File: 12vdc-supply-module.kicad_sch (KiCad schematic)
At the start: 1 part

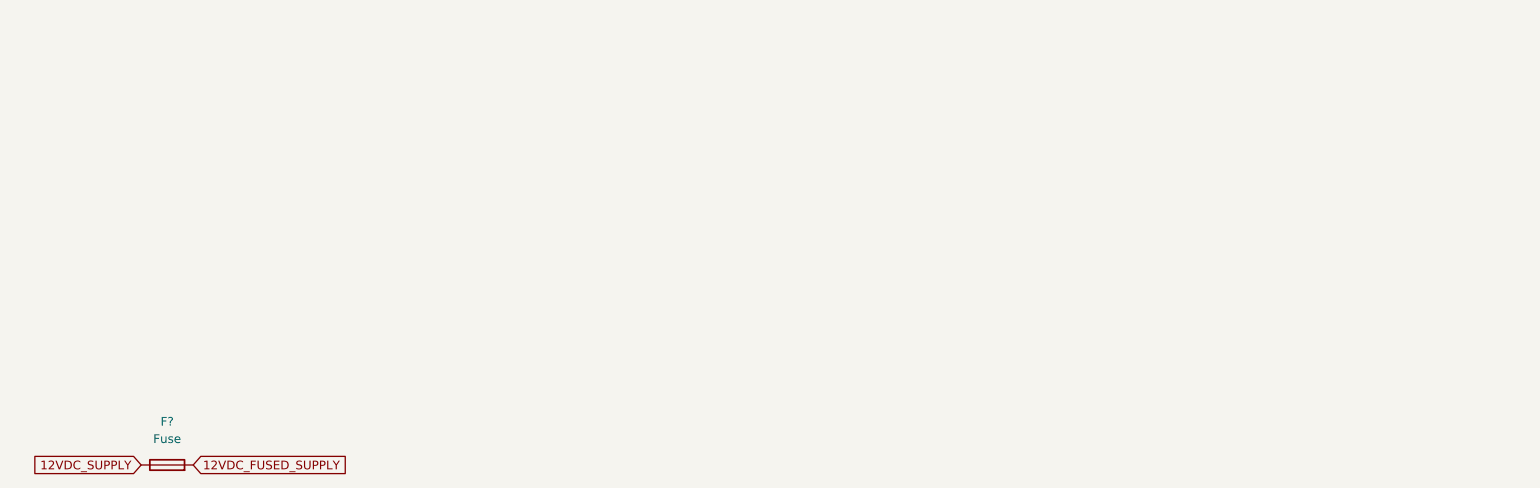
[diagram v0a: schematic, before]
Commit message: Draft 5VDC Supply Schematic
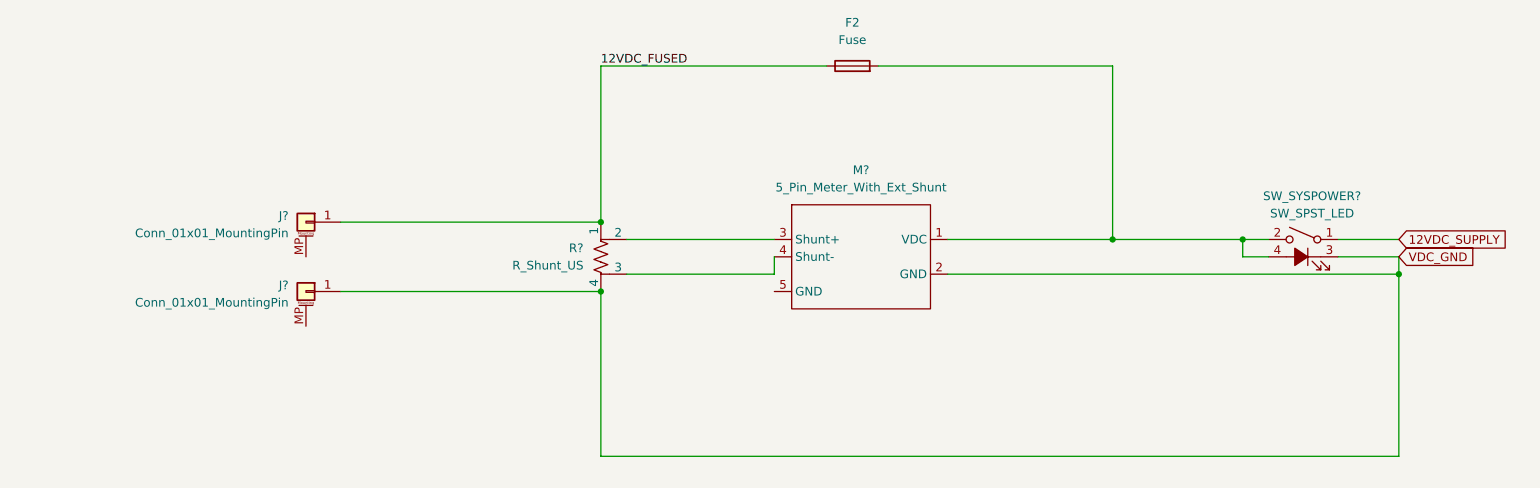
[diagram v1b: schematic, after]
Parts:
- added J? (x2): Conn_01x01_MountingPin, symbol Connector_Generic_MountingPin:Conn_01x01_MountingPin
- added M?: 5_Pin_Meter_With_Ext_Shunt, symbol bvm-library:5_Pin_Meter_With_Ext_Shunt
- added R?: R_Shunt_US, symbol Device:R_Shunt_US
- added SW_SYSPOWER?: SW_SPST_LED, symbol Switch:SW_SPST_LED
- gave numbers to parts that had none: 1
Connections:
- net 12VDC_SUPPLY: now also SW_SYSPOWER?.1; no longer F2.1
- net 12VDC_FUSED_SUPPLY: no longer names the net of F2.2
- net 12VDC_FUSED_SUPPLY: now also M?.1 (VDC), SW_SYSPOWER?.2, SW_SYSPOWER?.4 (A)
- new net: M?.3 (Shunt+), R?.2
- new net: M?.4 (Shunt-), R?.3
- new net 12VDC_FUSED: F2.1, J?.1 (Pin_1), R?.1
- new net VDC_GND: J?.1 (Pin_1), M?.2 (GND), R?.4, SW_SYSPOWER?.3 (K)
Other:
- moved on the sheet: F2
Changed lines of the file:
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@@
     (company "eatmellc")
   )
-  (global_label "12VDC_SUPPLY" (shape input) (at 68.58 82.55 180) (fields_autoplaced)
-    (effects (font (size 1.27 1.27)) (justify right))
-    (property "Intersheet References" "${INTERSHEET_REFS}" (id 0) (at 51.955 82.4706 0)
-      (effects (font (size 1.27 1.27)) (justify right))
-    )
+  (junction (at 135.89 46.99) (diameter 0) (color 0 0 0 0)
   )
-  (global_label "12VDC_FUSED_SUPPLY" (shape input) (at 76.2 82.55 0) (fields_autoplaced)
+  (junction (at 135.89 57.15) (diameter 0) (color 0 0 0 0)
+  )
+  (junction (at 229.87 49.53) (diameter 0) (color 0 0 0 0)
+  )
+  (junction (at 210.82 49.53) (diameter 0) (color 0 0 0 0)
+  )
+  (junction (at 252.73 54.61) (diameter 0) (color 0 0 0 0)
+  )
+  (wire (pts (xy 229.87 52.07) (xy 233.68 52.07))
+    (stroke (width 0) (type default) (color 0 0 0 0))
+  )
+  (wire (pts (xy 135.89 24.13) (xy 135.89 46.99))
+    (stroke (width 0) (type default) (color 0 0 0 0))
+  )
+  (wire (pts (xy 139.7 49.53) (xy 161.29 49.53))
+    (stroke (width 0) (type default) (color 0 0 0 0))
+  )
+  (wire (pts (xy 210.82 49.53) (xy 210.82 24.13))
+    (stroke (width 0) (type default) (color 0 0 0 0))
+  )
+  (wire (pts (xy 252.73 52.07) (xy 252.73 54.61))
+    (stroke (width 0) (type default) (color 0 0 0 0))
+  )
+  (wire (pts (xy 135.89 81.28) (xy 135.89 57.15))
+    (stroke (width 0) (type default) (color 0 0 0 0))
+  )
+  (wire (pts (xy 161.29 54.61) (xy 161.29 52.07))
+    (stroke (width 0) (type default) (color 0 0 0 0))
+  )
+  (wire (pts (xy 233.68 49.53) (xy 229.87 49.53))
+    (stroke (width 0) (type default) (color 0 0 0 0))
+  )
+  (wire (pts (xy 252.73 54.61) (xy 252.73 81.28))
+    (stroke (width 0) (type default) (color 0 0 0 0))
+  )
+  (wire (pts (xy 97.79 46.99) (xy 135.89 46.99))
+    (stroke (width 0) (type default) (color 0 0 0 0))
+  )
+  (wire (pts (xy 229.87 49.53) (xy 229.87 52.07))
+    (stroke (width 0) (type default) (color 0 0 0 0))
+  )
+  (wire (pts (xy 252.73 52.07) (xy 243.84 52.07))
+    (stroke (width 0) (type default) (color 0 0 0 0))
+  )
+  (wire (pts (xy 161.29 54.61) (xy 139.7 54.61))
+    (stroke (width 0) (type default) (color 0 0 0 0))
+  )
+  (wire (pts (xy 252.73 49.53) (xy 243.84 49.53))
+    (stroke (width 0) (type default) (color 0 0 0 0))
+  )
+  (wire (pts (xy 252.73 81.28) (xy 135.89 81.28))
+    (stroke (width 0) (type default) (color 0 0 0 0))
+  )
+  (wire (pts (xy 210.82 49.53) (xy 186.69 49.53))
+    (stroke (width 0) (type default) (color 0 0 0 0))
+  )
+  (wire (pts (xy 168.91 24.13) (xy 135.89 24.13))
+    (stroke (width 0) (type default) (color 0 0 0 0))
+  )
+  (wire (pts (xy 186.69 54.61) (xy 252.73 54.61))
+    (stroke (width 0) (type default) (color 0 0 0 0))
+  )
+  (wire (pts (xy 210.82 24.13) (xy 176.53 24.13))
+    (stroke (width 0) (type default) (color 0 0 0 0))
+  )
+  (wire (pts (xy 97.79 57.15) (xy 135.89 57.15))
+    (stroke (width 0) (type default) (color 0 0 0 0))
+  )
+  (wire (pts (xy 229.87 49.53) (xy 210.82 49.53))
+    (stroke (width 0) (type default) (color 0 0 0 0))
+  )
+  (label "12VDC_FUSED" (at 135.89 24.13 0)
+    (effects (font (size 1.27 1.27)) (justify left bottom))
+  )
+  (global_label "VDC_GND" (shape input) (at 252.73 52.07 0) (fields_autoplaced)
     (effects (font (size 1.27 1.27)) (justify left))
-    (property "Intersheet References" "${INTERSHEET_REFS}" (id 0) (at 99.8402 82.4706 0)
+    (property "Intersheet References" "${INTERSHEET_REFS}" (id 0) (at 263.6098 51.9906 0)
       (effects (font (size 1.27 1.27)) (justify left))
     )
   )
-  (symbol (lib_id "Device:Fuse") (at 72.39 82.55 90) (unit 1)
+  (global_label "12VDC_SUPPLY" (shape input) (at 252.73 49.53 0) (fields_autoplaced)
+    (effects (font (size 1.27 1.27)) (justify left))
+    (property "Intersheet References" "${INTERSHEET_REFS}" (id 0) (at 269.355 49.4506 0)
+      (effects (font (size 1.27 1.27)) (justify left))
+    )
+  )
+  (symbol (lib_id "bvm-library:5_Pin_Meter_With_Ext_Shunt") (at 168.91 54.61 0) (unit 1)
     (in_bom yes) (on_board yes) (fields_autoplaced)
-    (property "Reference" "F?" (id 0) (at 72.39 76.2 90))
-    (property "Value" "Fuse" (id 1) (at 72.39 78.74 90))
-    (property "Footprint" "" (id 2) (at 72.39 84.328 90)
+    (property "Reference" "M?" (id 0) (at 173.99 39.37 0))
+    (property "Value" "5_Pin_Meter_With_Ext_Shunt" (id 1) (at 173.99 41.91 0))
+    (property "Footprint" "" (id 2) (at 168.91 54.61 0)
       (effects (font (size 1.27 1.27)) hide)
     )
-    (property "Datasheet" "~" (id 3) (at 72.39 82.55 0)
+    (property "Datasheet" "" (id 3) (at 168.91 54.61 0)
+      (effects (font (size 1.27 1.27)) hide)
+    )
+    (pin "1")
+    (pin "2")
+    (pin "3")
+    (pin "4")
+    (pin "5")
+  )
+  (symbol (lib_id "Device:Fuse") (at 172.72 24.13 90) (unit 1)
+    (in_bom yes) (on_board yes) (fields_autoplaced)
+    (property "Reference" "F2" (id 0) (at 172.72 17.78 90))
+    (property "Value" "Fuse" (id 1) (at 172.72 20.32 90))
+    (property "Footprint" "" (id 2) (at 172.72 25.908 90)
+      (effects (font (size 1.27 1.27)) hide)
+    )
+    (property "Datasheet" "~" (id 3) (at 172.72 24.13 0)
       (effects (font (size 1.27 1.27)) hide)
     )
@@
     (pin "2")
   )
+  (symbol (lib_id "Device:R_Shunt_US") (at 135.89 52.07 0) (unit 1)
+    (in_bom yes) (on_board yes) (fields_autoplaced)
+    (property "Reference" "R?" (id 0) (at 133.35 50.7999 0)
+      (effects (font (size 1.27 1.27)) (justify right))
+    )
+    (property "Value" "R_Shunt_US" (id 1) (at 133.35 53.3399 0)
+      (effects (font (size 1.27 1.27)) (justify right))
+    )
+    (property "Footprint" "" (id 2) (at 134.112 52.07 90)
+      (effects (font (size 1.27 1.27)) hide)
+    )
+    (property "Datasheet" "~" (id 3) (at 135.89 52.07 0)
+      (effects (font (size 1.27 1.27)) hide)
+    )
+    (pin "1")
+    (pin "2")
+    (pin "3")
+    (pin "4")
+  )
+  (symbol (lib_id "Switch:SW_SPST_LED") (at 238.76 52.07 0) (mirror y) (unit 1)
+    (in_bom yes) (on_board yes) (fields_autoplaced)
+    (property "Reference" "SW_SYSPOWER?" (id 0) (at 240.03 43.18 0))
+    (property "Value" "SW_SPST_LED" (id 1) (at 240.03 45.72 0))
+    (property "Footprint" "" (id 2) (at 238.76 44.45 0)
+      (effects (font (size 1.27 1.27)) hide)
+    )
+    (property "Datasheet" "~" (id 3) (at 238.76 44.45 0)
+      (effects (font (size 1.27 1.27)) hide)
+    )
+    (pin "1")
+    (pin "2")
+    (pin "3")
+    (pin "4")
+  )
+  (symbol (lib_id "Connector_Generic_MountingPin:Conn_01x01_MountingPin") (at 92.71 57.15 0) (mirror y) (unit 1)
+    (in_bom yes) (on_board yes) (fields_autoplaced)
+    (property "Reference" "J?" (id 0) (at 90.17 56.2355 0)
+      (effects (font (size 1.27 1.27)) (justify left))
+    )
+    (property "Value" "Conn_01x01_MountingPin" (id 1) (at 90.17 58.7755 0)
+      (effects (font (size 1.27 1.27)) (justify left))
+    )
+    (property "Footprint" "" (id 2) (at 92.71 57.15 0)
+      (effects (font (size 1.27 1.27)) hide)
+    )
+    (property "Datasheet" "~" (id 3) (at 92.71 57.15 0)
+      (effects (font (size 1.27 1.27)) hide)
+    )
+    (pin "1")
+    (pin "MP")
+  )
+  (symbol (lib_id "Connector_Generic_MountingPin:Conn_01x01_MountingPin") (at 92.71 46.99 0) (mirror y) (unit 1)
+    (in_bom yes) (on_board yes) (fields_autoplaced)
+    (property "Reference" "J?" (id 0) (at 90.17 46.0755 0)
+      (effects (font (size 1.27 1.27)) (justify left))
+    )
+    (property "Value" "Conn_01x01_MountingPin" (id 1) (at 90.17 48.6155 0)
+      (effects (font (size 1.27 1.27)) (justify left))
+    )
+    (property "Footprint" "" (id 2) (at 92.71 46.99 0)
+      (effects (font (size 1.27 1.27)) hide)
+    )
+    (property "Datasheet" "~" (id 3) (at 92.71 46.99 0)
+      (effects (font (size 1.27 1.27)) hide)
+    )
+    (pin "1")
+    (pin "MP")
+  )
 )
